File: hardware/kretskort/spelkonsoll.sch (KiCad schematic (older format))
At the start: 18 parts, among them SW1 SW_Push, SW2 SW_Push, SW3 SW_Push, SW4 SW_Push, SW5 SW_Push, SW6 SW_Push, SW7 SW_Push, SW8 SW_Push, U1 ESP32-DEVKITC-32D, U2 ILI9488

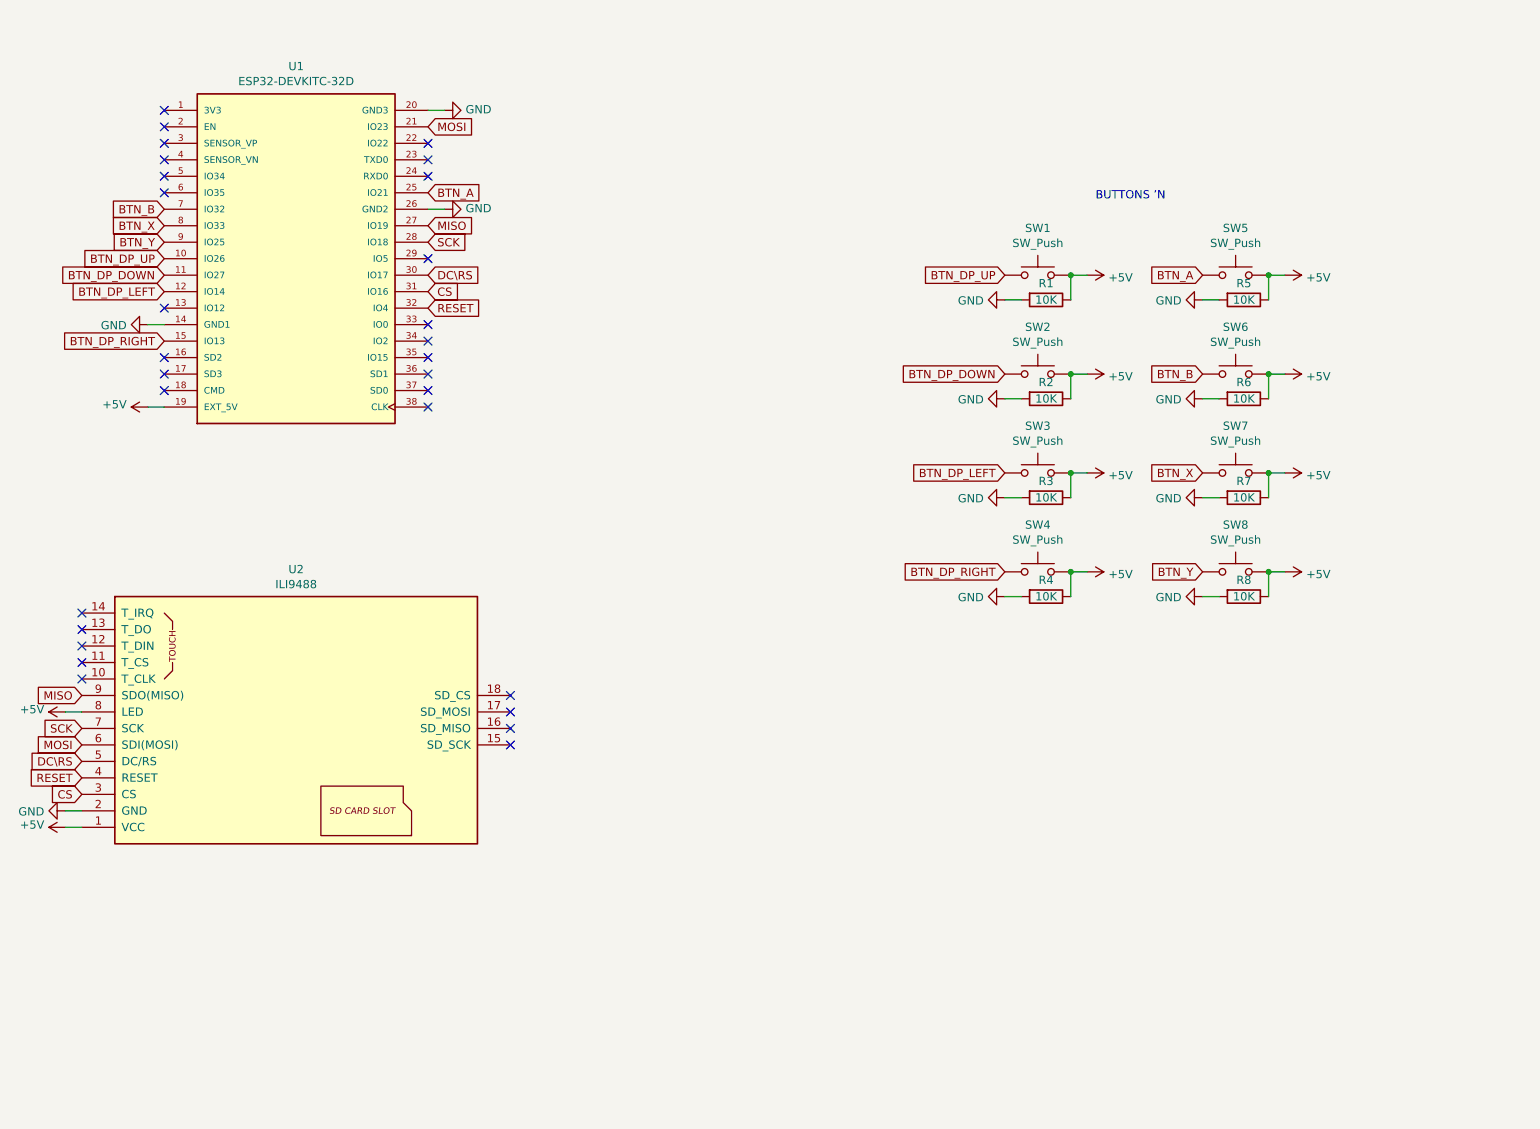
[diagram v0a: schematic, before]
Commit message: update KiCad files
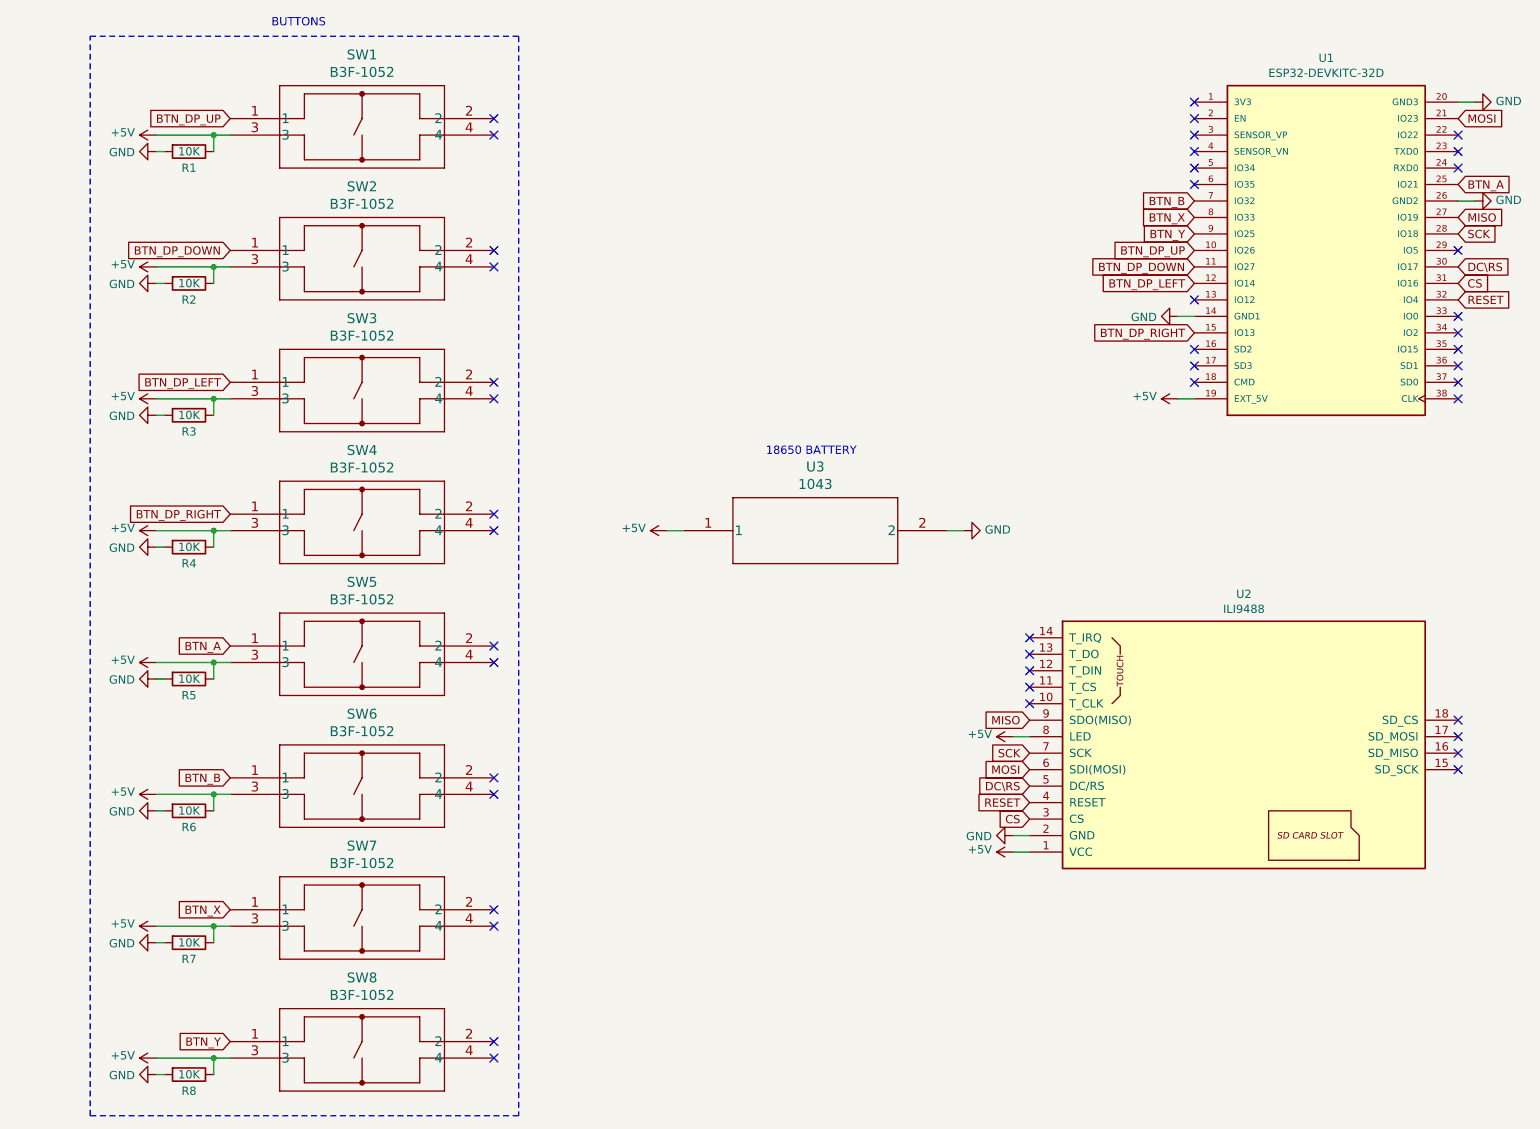
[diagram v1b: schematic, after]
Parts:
- removed SW1, SW2, SW3, SW4, SW5, SW6, SW7, SW8: SW_Push, footprints:B3F1052, symbol spelkonsoll-rescue:SW_Push-Switch
- added SW1, SW2, SW3, SW4, SW5, SW6, SW7, SW8: B3F-1052, footprints:Button, symbol Button:B3F-1052
- added U3: 1043, footprints:18650holder, symbol 18650holder:1043
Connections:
- net +5V: now also SW1.3, SW2.3, SW3.3, SW4.3, SW5.3, SW6.3, SW7.3, SW8.3, U3.1
- net BTN_A: now also SW5.1
- net BTN_B: now also SW6.1
- net BTN_DP_DOWN: now also SW2.1
- net BTN_DP_LEFT: now also SW3.1
- net BTN_DP_RIGHT: now also SW4.1
- net BTN_DP_UP: now also SW1.1
- net BTN_X: now also SW7.1
- net BTN_Y: now also SW8.1
- net GND: now also U3.2
- no-connect marks 29 -> 45
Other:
- note added: "18650 BATTERY"
- note added: "BUTTONS"
- note removed: "BUTTONS ’N"
- moved on the sheet: R1, U1, U2
